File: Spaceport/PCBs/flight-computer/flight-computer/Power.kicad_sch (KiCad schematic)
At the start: 26 parts, among them IC1 AP7362-33SP-13, IC2 AP7362-33SP-13, J10 Conn_01x02, J9 Conn_01x02, U6 TPS62A03DRLR

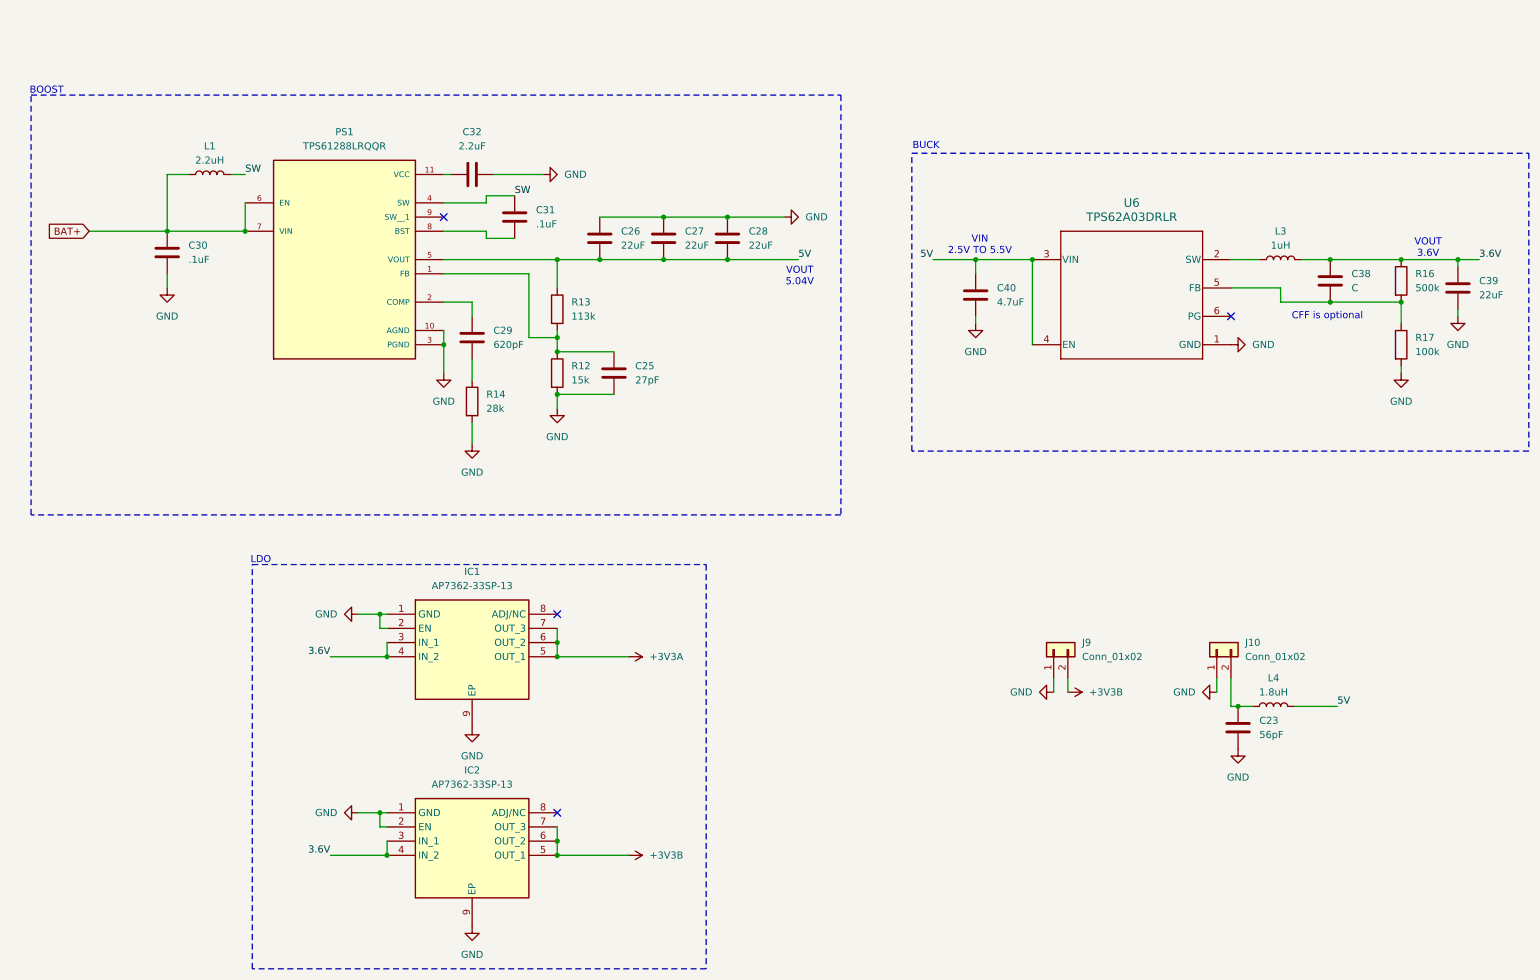
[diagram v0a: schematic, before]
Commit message: removed SdCard
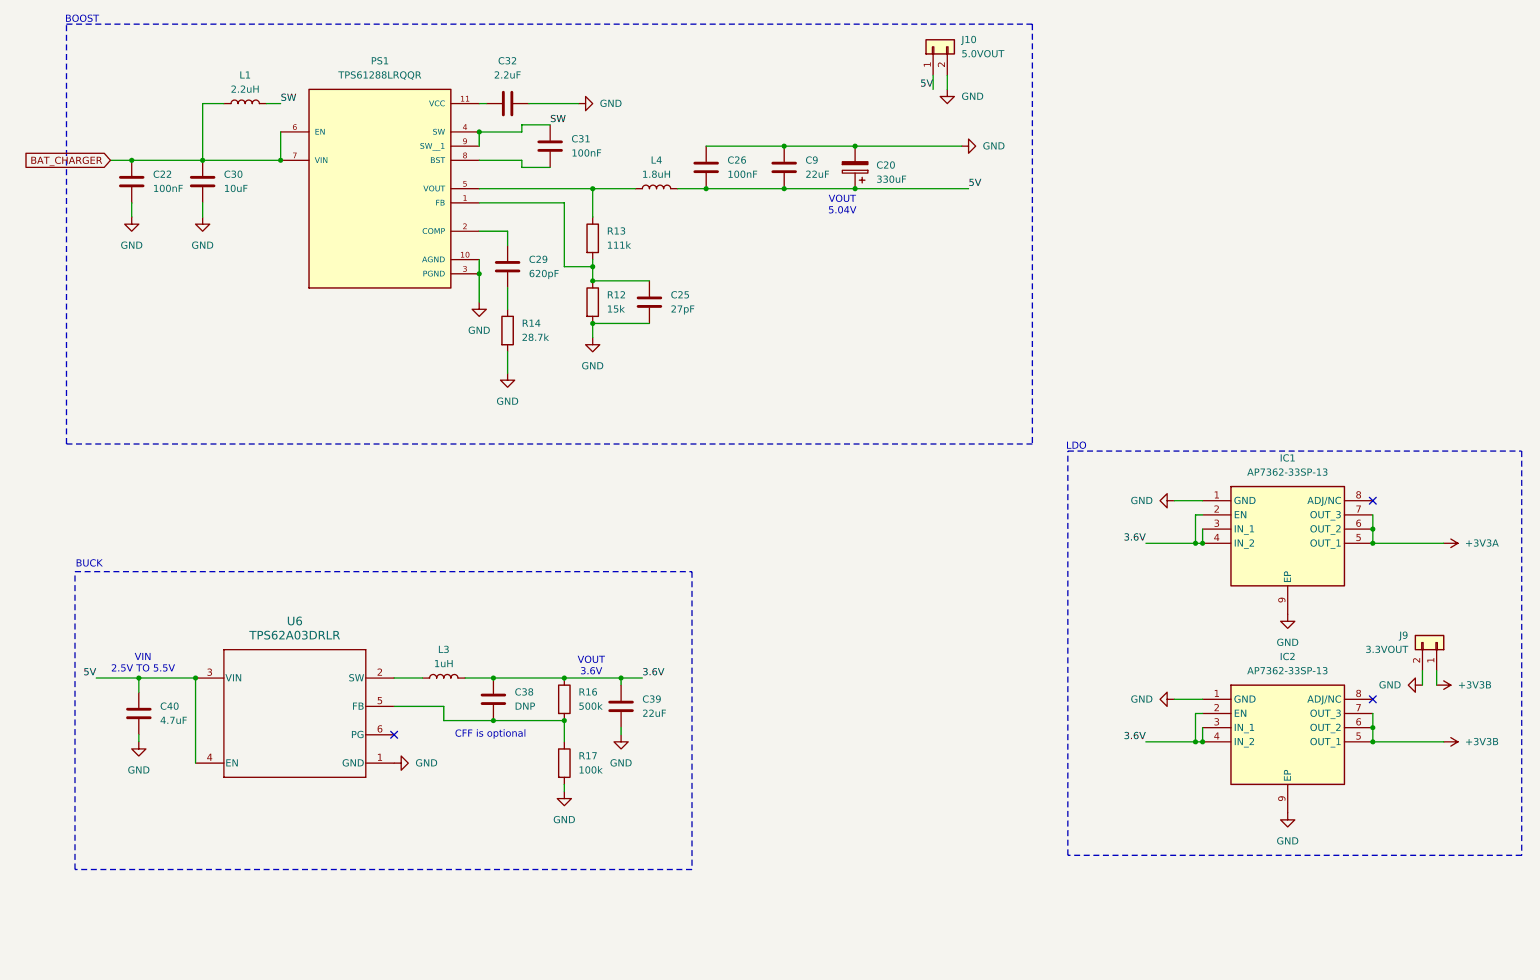
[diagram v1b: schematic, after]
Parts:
- removed C23: 56pF, symbol Device:C
- removed C27, C28: 22uF, symbol Device:C
- added C20: 330uF, symbol Device:C_Polarized
- added C22: 100nF, symbol Device:C
- added C9: 22uF, symbol Device:C
- C26: value 22uF -> 100nF
- C30: value .1uF -> 10uF
- C31: value .1uF -> 100nF
- C38: value C -> DNP
- J10: value Conn_01x02 -> 5.0VOUT
- J9: value Conn_01x02 -> 3.3VOUT
- R13: value 113k -> 111k
- R14: value 28k -> 28.7k
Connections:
- net +3V3B: now also J9.1 (Pin_1); no longer J9.2 (Pin_2)
- net 3.6V: now also IC1.2 (EN), IC2.2 (EN)
- net 5V: now also J10.1 (Pin_1), C20.1, C9.2; no longer PS1.5 (VOUT), R13.1
- net GND: now also J10.2 (Pin_2), J9.2 (Pin_2), C20.2, C22.2, C9.1; no longer IC1.2 (EN), IC2.2 (EN), J10.1 (Pin_1), J9.1 (Pin_1)
- net SW: now also PS1.9 (SW__1)
- net at L4.1: now also PS1.5 (VOUT), R13.1; no longer J10.2 (Pin_2)
- net BAT+ renamed BAT_CHARGER
- net BAT_CHARGER: now also C22.1
- no-connect marks 4 -> 3
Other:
- moved on the sheet: C25, C26, C29, C30, C31, C32, C38, C39, C40, IC1, IC2, J10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
